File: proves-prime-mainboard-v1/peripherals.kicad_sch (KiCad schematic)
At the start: 19 parts, among them IC3 RV-3028-C7_32.768kHz_1ppm_TA_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, J8 Molex 503398-1892, U11 MCP9808T-E/MS, U5 LSM6DSOTR, U6 LSM303AGRTR

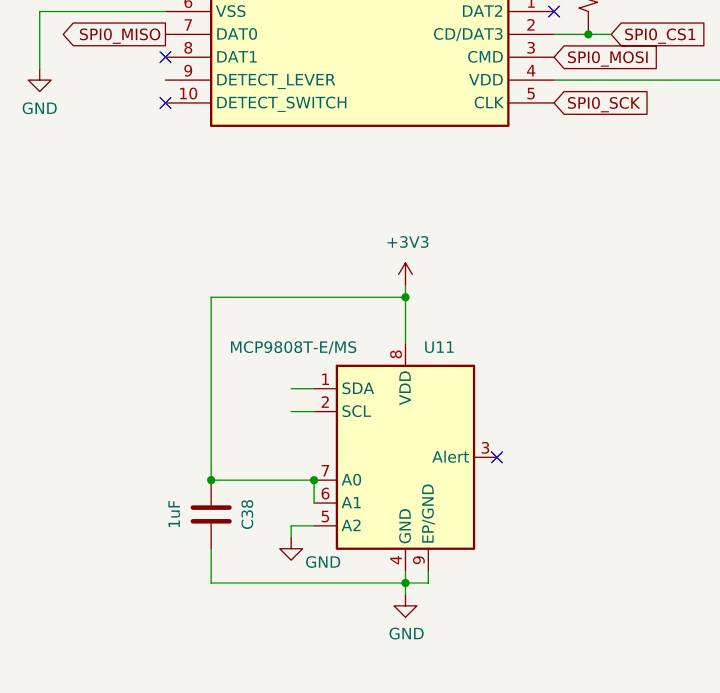
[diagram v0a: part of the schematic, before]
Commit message: More Wiring!
Connected Additional Peripheral
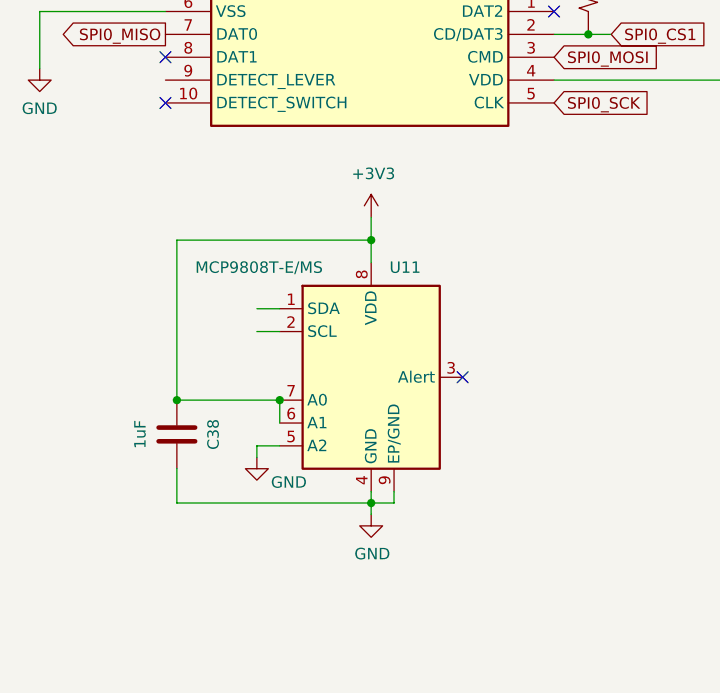
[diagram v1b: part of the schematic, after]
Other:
- moved on the sheet: C38, U11
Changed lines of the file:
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@@
 	(paper "A4")
 	(junction
-		(at 67.31 106.68)
+		(at 63.5 97.79)
 		(diameter 0)
 		(color 0 0 0 0)
@@
 	)
 	(junction
-		(at 45.72 95.25)
+		(at 41.91 86.36)
 		(diameter 0)
 		(color 0 0 0 0)
@@
 	)
 	(junction
-		(at 57.15 95.25)
+		(at 63.5 68.58)
 		(diameter 0)
 		(color 0 0 0 0)
 	)
 	(junction
-		(at 237.998 26.797)
+		(at 53.34 86.36)
 		(diameter 0)
 		(color 0 0 0 0)
 	)
 	(junction
-		(at 171.45 46.99)
+		(at 237.998 26.797)
 		(diameter 0)
 		(color 0 0 0 0)
 	)
 	(junction
-		(at 213.36 110.49)
+		(at 171.45 46.99)
 		(diameter 0)
 		(color 0 0 0 0)
 	)
 	(junction
-		(at 67.31 74.93)
+		(at 213.36 110.49)
 		(diameter 0)
 		(color 0 0 0 0)
@@
 	)
 	(no_connect
-		(at 77.47 92.71)
+		(at 73.66 83.82)
 	)
 	(no_connect
@@
 	(wire
 		(pts
-			(xy 54.61 85.09) (xy 57.15 85.09)
+			(xy 50.8 76.2) (xy 53.34 76.2)
 		)
 		(stroke
@@
 	(wire
 		(pts
-			(xy 69.85 105.41) (xy 69.85 106.68)
+			(xy 66.04 96.52) (xy 66.04 97.79)
 		)
 		(stroke
@@
 	(wire
 		(pts
-			(xy 45.72 74.93) (xy 45.72 95.25)
+			(xy 41.91 68.58) (xy 41.91 86.36)
 		)
 		(stroke
@@
 	(wire
 		(pts
-			(xy 54.61 87.63) (xy 57.15 87.63)
+			(xy 50.8 78.74) (xy 53.34 78.74)
 		)
 		(stroke
@@
 	(wire
 		(pts
-			(xy 45.72 106.68) (xy 67.31 106.68)
+			(xy 41.91 97.79) (xy 63.5 97.79)
 		)
 		(stroke
@@
 	(wire
 		(pts
+			(xy 63.5 66.04) (xy 63.5 68.58)
+		)
+		(stroke
+			(width 0)
+			(type default)
+		)
+	)
+	(wire
+		(pts
 			(xy 264.16 54.61) (xy 273.05 54.61)
 		)
@@
 	(wire
 		(pts
-			(xy 57.15 95.25) (xy 45.72 95.25)
+			(xy 53.34 86.36) (xy 41.91 86.36)
 		)
 		(stroke
@@
 	(wire
 		(pts
-			(xy 67.31 106.68) (xy 67.31 107.95)
+			(xy 63.5 97.79) (xy 63.5 99.06)
 		)
 		(stroke
@@
 	(wire
 		(pts
-			(xy 57.15 100.33) (xy 54.61 100.33)
+			(xy 53.34 91.44) (xy 50.8 91.44)
 		)
 		(stroke
@@
 	(wire
 		(pts
-			(xy 57.15 95.25) (xy 57.15 97.79)
+			(xy 53.34 86.36) (xy 53.34 88.9)
 		)
 		(stroke
@@
 	(wire
 		(pts
-			(xy 45.72 106.68) (xy 45.72 102.87)
+			(xy 41.91 97.79) (xy 41.91 93.98)
 		)
 		(stroke
@@
 	(wire
 		(pts
-			(xy 67.31 106.68) (xy 67.31 105.41)
+			(xy 63.5 97.79) (xy 63.5 96.52)
 		)
 		(stroke
@@
 	(wire
 		(pts
-			(xy 67.31 74.93) (xy 67.31 80.01)
+			(xy 83.82 50.8) (xy 104.14 50.8)
 		)
 		(stroke
@@
 	(wire
 		(pts
-			(xy 83.82 50.8) (xy 104.14 50.8)
+			(xy 171.45 46.99) (xy 171.45 50.8)
 		)
 		(stroke
@@
 	(wire
 		(pts
-			(xy 171.45 46.99) (xy 171.45 50.8)
+			(xy 50.8 91.44) (xy 50.8 92.71)
 		)
 		(stroke
@@
 	(wire
 		(pts
-			(xy 54.61 100.33) (xy 54.61 101.6)
+			(xy 63.5 68.58) (xy 63.5 71.12)
 		)
 		(stroke
@@
 	(wire
 		(pts
-			(xy 69.85 106.68) (xy 67.31 106.68)
+			(xy 66.04 97.79) (xy 63.5 97.79)
 		)
 		(stroke
@@
 	(wire
 		(pts
-			(xy 67.31 73.66) (xy 67.31 74.93)
-		)
-		(stroke
-			(width 0)
-			(type default)
-		)
-	)
-	(wire
-		(pts
 			(xy 267.97 95.25) (xy 267.97 78.74)
 		)
@@
 	(wire
 		(pts
-			(xy 45.72 74.93) (xy 67.31 74.93)
+			(xy 41.91 68.58) (xy 63.5 68.58)
 		)
 		(stroke
@@
 	(symbol
 		(lib_id "Sensor_Temperature:MCP9808_DFN")
-		(at 67.31 92.71 0)
+		(at 63.5 83.82 0)
 		(unit 1)
 		(exclude_from_sim no)
@@
 		(dnp no)
 		(property "Reference" "U11"
-			(at 69.342 80.518 0)
+			(at 65.532 71.628 0)
 			(effects
 				(font
@@
 		)
 		(property "Value" "MCP9808T-E/MS"
-			(at 47.752 80.518 0)
+			(at 43.942 71.628 0)
 			(effects
 				(font
@@
 		)
 		(property "Footprint" "Package_SO:MSOP-8-1EP_3x3mm_P0.65mm_EP1.5x1.8mm_ThermalVias"
-			(at 67.31 92.71 0)
+			(at 63.5 83.82 0)
 			(effects
 				(font
@@
 		)
 		(property "Datasheet" "http://ww1.microchip.com/downloads/en/DeviceDoc/MCP9808-0.5C-Maximum-Accuracy-Digital-Temperature-Sensor-Data-Sheet-DS20005095B.pdf"
-			(at 60.96 81.28 0)
+			(at 57.15 72.39 0)
 			(effects
 				(font
@@
 		)
 		(property "Description" ""
-			(at 67.31 92.71 0)
+			(at 63.5 83.82 0)
 			(effects
 				(font
@@
 	(symbol
 		(lib_id "solar-panel-side-Z-rescue:+3.3V-power")
-		(at 67.31 73.66 0)
+		(at 63.5 66.04 0)
 		(unit 1)
 		(exclude_from_sim no)
@@
 		(dnp no)
 		(property "Reference" "#PWR078"
-			(at 67.31 77.47 0)
+			(at 63.5 69.85 0)
 			(effects
 				(font
@@
 		)
 		(property "Value" "+3V3"
-			(at 67.564 68.834 0)
+			(at 63.754 61.214 0)
 			(effects
 				(font
@@
 		)
 		(property "Footprint" ""
-			(at 67.31 73.66 0)
+			(at 63.5 66.04 0)
 			(effects
 				(font
@@
 		)
 		(property "Datasheet" ""
-			(at 67.31 73.66 0)
+			(at 63.5 66.04 0)
 			(effects
 				(font
@@
 		)
 		(property "Description" ""
-			(at 67.31 73.66 0)
+			(at 63.5 66.04 0)
 			(effects
 				(font
@@
 	(symbol
 		(lib_id "power:GND")
-		(at 67.31 107.95 0)
+		(at 63.5 99.06 0)
 		(unit 1)
 		(exclude_from_sim no)
@@
 		(dnp no)
 		(property "Reference" "#PWR079"
-			(at 67.31 114.3 0)
+			(at 63.5 105.41 0)
 			(effects
 				(font
@@
 		)
 		(property "Value" "GND"
-			(at 67.437 112.3442 0)
+			(at 63.627 103.4542 0)
 			(effects
 				(font
@@
 		)
 		(property "Footprint" ""
-			(at 67.31 107.95 0)
+			(at 63.5 99.06 0)
 			(effects
 				(font
@@
 		)
 		(property "Datasheet" ""
-			(at 67.31 107.95 0)
+			(at 63.5 99.06 0)
 			(effects
 				(font
@@
 		)
 		(property "Description" ""
-			(at 67.31 107.95 0)
+			(at 63.5 99.06 0)
 			(effects
 				(font
@@
 	(symbol
 		(lib_id "Device:C")
-		(at 45.72 99.06 0)
+		(at 41.91 90.17 0)
 		(unit 1)
 		(exclude_from_sim no)
@@
 		(dnp no)
 		(property "Reference" "C38"
-			(at 49.784 99.06 90)
+			(at 45.974 90.17 90)
 			(effects
 				(font
@@
 		)
 		(property "Value" "1uF"
-			(at 41.656 99.06 90)
+			(at 37.846 90.17 90)
 			(effects
 				(font
@@
 		)
 		(property "Footprint" "Capacitor_SMD:C_0805_2012Metric"
-			(at 46.6852 102.87 0)
+			(at 42.8752 93.98 0)
 			(effects
 				(font
@@
 		)
 		(property "Datasheet" "~"
-			(at 45.72 99.06 0)
+			(at 41.91 90.17 0)
 			(effects
 				(font
@@
 		)
 		(property "Description" ""
-			(at 45.72 99.06 0)
+			(at 41.91 90.17 0)
 			(effects
 				(font
@@
 	(symbol
 		(lib_id "power:GND")
-		(at 54.61 101.6 0)
+		(at 50.8 92.71 0)
 		(unit 1)
 		(exclude_from_sim no)
@@
 		(dnp no)
 		(property "Reference" "#PWR077"
-			(at 54.61 107.95 0)
+			(at 50.8 99.06 0)
 			(effects
 				(font
@@
 		)
 		(property "Value" "GND"
-			(at 58.166 104.394 0)
+			(at 54.356 95.504 0)
 			(effects
 				(font
@@
 		)
 		(property "Footprint" ""
-			(at 54.61 101.6 0)
+			(at 50.8 92.71 0)
 			(effects
 				(font
@@
 		)
 		(property "Datasheet" ""
-			(at 54.61 101.6 0)
+			(at 50.8 92.71 0)
 			(effects
 				(font
@@
 		)
 		(property "Description" ""
-			(at 54.61 101.6 0)
+			(at 50.8 92.71 0)
 			(effects
 				(font
